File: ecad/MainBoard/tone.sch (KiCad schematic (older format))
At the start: 5 parts, among them IC1 RC4558

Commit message: Update BOM and SPIRCE SIM
Add netlist to calculate power dissipation through each resistor
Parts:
- C9: MPN (none) -> 12065C204KAT4A
- IC1: Digi-Key_PN (none) -> 296-9650-5-ND; MPN (none) -> RC4558D
- R11: Digi-Key_PN (none) -> PT220XTR-ND; MPN (none) -> ERJ-1TYJ221U
- R17: Digi-Key_PN (none) -> A130048TR-ND; MPN (none) -> CRGCQ0402J1K0
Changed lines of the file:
@@
 F 1 "220n" V 1000 1600 50  0000 C CNN
 F 2 "Capacitor_SMD:C_0805_2012Metric_Pad1.18x1.45mm_HandSolder" H 1188 1450 50  0001 C CNN
-F 3 "~" H 1150 1600 50  0001 C CNN
+F 3 "https://datasheets.avx.com/X7RDielectric.pdf" H 1150 1600 50  0001 C CNN
+F 4 "12065C204KAT4A" H 1150 1600 50  0001 C CNN "MPN"
 	1    1150 1600
 	0    -1   -1   0
@@
 F 2 "Resistor_SMD:R_0805_2012Metric_Pad1.20x1.40mm_HandSolder" V 1430 1600 50  0001 C CNN
 F 3 "~" H 1500 1600 50  0001 C CNN
+F 4 "PT220XTR-ND" H 1500 1600 50  0001 C CNN "Digi-Key_PN"
+F 5 "ERJ-1TYJ221U" H 1500 1600 50  0001 C CNN "MPN"
 	1    1500 1600
 	0    -1   -1   0
@@
 F 2 "Resistor_SMD:R_0805_2012Metric_Pad1.20x1.40mm_HandSolder" V 1530 1200 50  0001 C CNN
 F 3 "~" H 1600 1200 50  0001 C CNN
+F 4 "A130048TR-ND" H 1600 1200 50  0001 C CNN "Digi-Key_PN"
+F 5 "CRGCQ0402J1K0" H 1600 1200 50  0001 C CNN "MPN"
 	1    1600 1200
 	0    1    1    0
@@
 F 6 "Y" H 1550 850 50  0001 C CNN "Spice_Netlist_Enabled"
 F 7 "../lib/spice_models/RC4558.301.lib" H 1550 850 50  0001 C CNN "Spice_Lib_File"
+F 8 "296-9650-5-ND" H 1550 850 50  0001 C CNN "Digi-Key_PN"
+F 9 "RC4558D" H 1550 850 50  0001 C CNN "MPN"
 	2    1550 850
 	1    0    0    -1

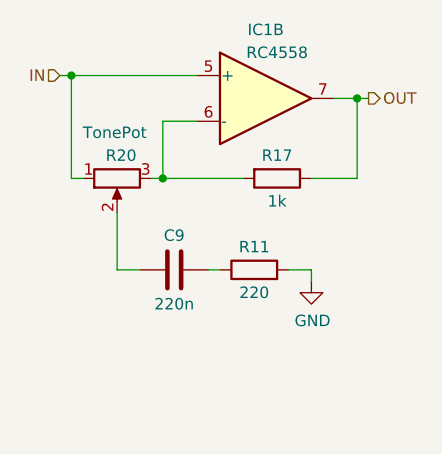
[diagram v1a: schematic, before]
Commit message: Clean up ecad
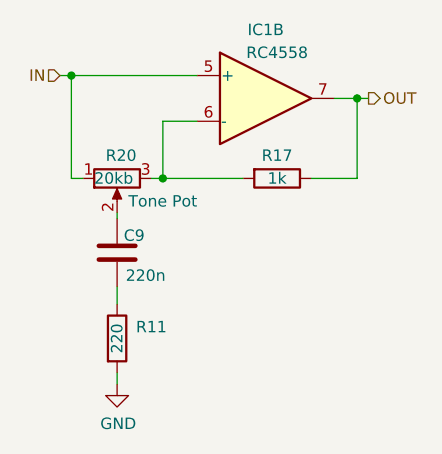
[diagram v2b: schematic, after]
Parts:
- C9: footprint Capacitor_SMD:C_0805_2012Metric_Pad1.18x1.45mm_HandSolder -> Capacitor_SMD:C_1206_3216Metric_Pad1.33x1.80mm_HandSolder; Digi-Key_PN (none) -> 478-12065C204KAT4ADKR-ND
- IC1: footprint Package_SO:Texas_R-PDSO-G8_EP2.95x4.9mm_Mask2.4x3.1mm -> DigiKey:SOIC-8_W3.9mm
- R11: footprint Resistor_SMD:R_0805_2012Metric_Pad1.20x1.40mm_HandSolder -> Resistor_SMD:R_2512_6332Metric_Pad1.40x3.35mm_HandSolder
- R17: footprint Resistor_SMD:R_0805_2012Metric_Pad1.20x1.40mm_HandSolder -> Resistor_SMD:R_0402_1005Metric_Pad0.72x0.64mm_HandSolder
- R20: value TonePot -> 20kb; Category (none) -> Tone Pot; Digi-Key_PN (none) -> 75160-195-08LF; Spice_Lib_File ../lib/spice_models/pot.lib -> ../lib/spice_models/pots.lib
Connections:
- net at R20.2: now also C9.2; no longer C9.1
- net at R11.1: now also C9.1; no longer C9.2
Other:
- moved on the sheet: C9, R11
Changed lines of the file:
@@
 encoding utf-8
 Sheet 3 5
-Title "Effects Board"
-Date "2021-01-17"
-Rev "1.0"
-Comp "Panda Pals"
-Comment1 "John McAvoy"
+Title "Screaming Panda Guitar Pedal"
+Date "2021-08-08"
+Rev "1v0"
+Comp "John McAvoy"
+Comment1 ""
 Comment2 ""
 Comment3 ""
@@
 L Device:C C?
 U 1 1 6027E33E
-P 1150 1600
+P 900 1525
 AR Path="/6027E33E" Ref="C?"  Part="1"
 AR Path="/60307048/6027E33E" Ref="C9"  Part="1"
-F 0 "C9" V 1300 1600 50  0000 C CNN
-F 1 "220n" V 1000 1600 50  0000 C CNN
-F 2 "Capacitor_SMD:C_0805_2012Metric_Pad1.18x1.45mm_HandSolder" H 1188 1450 50  0001 C CNN
-F 3 "https://datasheets.avx.com/X7RDielectric.pdf" H 1150 1600 50  0001 C CNN
-F 4 "12065C204KAT4A" H 1150 1600 50  0001 C CNN "MPN"
-	1    1150 1600
-	0    -1   -1   0
+F 0 "C9" H 825 1450 50  0000 C CNN
+F 1 "220n" H 775 1625 50  0000 C CNN
+F 2 "Capacitor_SMD:C_1206_3216Metric_Pad1.33x1.80mm_HandSolder" H 938 1375 50  0001 C CNN
+F 3 "https://datasheets.avx.com/X7RDielectric.pdf" H 900 1525 50  0001 C CNN
+F 4 "12065C204KAT4A" H 900 1525 50  0001 C CNN "MPN"
+F 5 "478-12065C204KAT4ADKR-ND" H 900 1525 50  0001 C CNN "Digi-Key_PN"
+	1    900  1525
+	-1   0    0    1
 $EndComp
 $Comp
 L Device:R R?
 U 1 1 6027E344
-P 1500 1600
+P 900 1900
 AR Path="/6027E344" Ref="R?"  Part="1"
 AR Path="/60307048/6027E344" Ref="R11"  Part="1"
-F 0 "R11" V 1600 1600 50  0000 C CNN
-F 1 "220" V 1400 1600 50  0000 C CNN
-F 2 "Resistor_SMD:R_0805_2012Metric_Pad1.20x1.40mm_HandSolder" V 1430 1600 50  0001 C CNN
-F 3 "~" H 1500 1600 50  0001 C CNN
-F 4 "PT220XTR-ND" H 1500 1600 50  0001 C CNN "Digi-Key_PN"
-F 5 "ERJ-1TYJ221U" H 1500 1600 50  0001 C CNN "MPN"
-	1    1500 1600
-	0    -1   -1   0
+F 0 "R11" H 1050 1950 50  0000 C CNN
+F 1 "220" V 900 1900 50  0000 C CNN
+F 2 "Resistor_SMD:R_2512_6332Metric_Pad1.40x3.35mm_HandSolder" V 830 1900 50  0001 C CNN
+F 3 "https://b2b-api.panasonic.eu/file_stream/pids/fileversion/1242" H 900 1900 50  0001 C CNN
+F 4 "PT220XTR-ND" H 900 1900 50  0001 C CNN "Digi-Key_PN"
+F 5 "ERJ-1TYJ221U" H 900 1900 50  0001 C CNN "MPN"
+	1    900  1900
+	1    0    0    -1
 $EndComp
-Wire Wire Line
-	1300 1600 1350 1600
 Text HLabel 2000 850  2    50   Output ~ 0
 OUT
@@
 AR Path="/60307048/6027E362" Ref="R17"  Part="1"
 F 0 "R17" V 1500 1200 50  0000 C CNN
-F 1 "1k" V 1700 1200 50  0000 C CNN
-F 2 "Resistor_SMD:R_0805_2012Metric_Pad1.20x1.40mm_HandSolder" V 1530 1200 50  0001 C CNN
-F 3 "~" H 1600 1200 50  0001 C CNN
+F 1 "1k" V 1600 1200 50  0000 C CNN
+F 2 "Resistor_SMD:R_0402_1005Metric_Pad0.72x0.64mm_HandSolder" V 1530 1200 50  0001 C CNN
+F 3 "https://www.te.com/commerce/DocumentDelivery/DDEController?Action=srchrtrv&DocNm=1773204-3&DocType=DS&DocLang=English" H 1600 1200 50  0001 C CNN
 F 4 "A130048TR-ND" H 1600 1200 50  0001 C CNN "Digi-Key_PN"
 F 5 "CRGCQ0402J1K0" H 1600 1200 50  0001 C CNN "MPN"
@@
 F 0 "IC1" H 1550 1150 50  0000 C CNN
 F 1 "RC4558" H 1600 1050 50  0000 C CNN
-F 2 "Package_SO:Texas_R-PDSO-G8_EP2.95x4.9mm_Mask2.4x3.1mm" H 1550 850 50  0001 C CNN
+F 2 "DigiKey:SOIC-8_W3.9mm" H 1550 850 50  0001 C CNN
 F 3 "http://www.ti.com/lit/ds/symlink/rc4558.pdf" H 1550 850 50  0001 C CNN
 F 4 "X" H 1550 850 50  0001 C CNN "Spice_Primitive"
@@
 P 900 1200
 F 0 "R20" V 800 1250 50  0000 R CNN
-F 1 "TonePot" V 700 1350 50  0000 R CNN
+F 1 "20kb" V 900 1300 50  0000 R CNN
 F 2 "Connector_PinHeader_2.54mm:PinHeader_1x03_P2.54mm_Vertical" H 900 1200 50  0001 C CNN
-F 3 "~" H 900 1200 50  0001 C CNN
+F 3 "https://www.bourns.com/docs/Product-Datasheets/PTV09.pdf" H 900 1200 50  0001 C CNN
 F 4 "X" H 900 1200 50  0001 C CNN "Spice_Primitive"
 F 5 "POTTone" H 900 1200 50  0001 C CNN "Spice_Model"
 F 6 "Y" H 900 1200 50  0001 C CNN "Spice_Netlist_Enabled"
-F 7 "../lib/spice_models/pot.lib" H 900 1200 50  0001 C CNN "Spice_Lib_File"
+F 7 "../lib/spice_models/pots.lib" H 900 1200 50  0001 C CNN "Spice_Lib_File"
+F 8 "Tone Pot" V 1000 1000 50  0000 C CNN "Category"
+F 9 "75160-195-08LF" H 900 1200 50  0001 C CNN "Digi-Key_PN"
+F 10 "" H 900 1200 50  0001 C CNN "MPN"
 	1    900  1200
 	0    -1   1    0
@@
 L power:GND #PWR?
 U 1 1 6027E34B
-P 1750 1650
+P 900 2100
 AR Path="/6027E34B" Ref="#PWR?"  Part="1"
 AR Path="/60307048/6027E34B" Ref="#PWR017"  Part="1"
-F 0 "#PWR017" H 1750 1400 50  0001 C CNN
-F 1 "GND" H 1755 1477 50  0000 C CNN
-F 2 "" H 1750 1650 50  0001 C CNN
-F 3 "" H 1750 1650 50  0001 C CNN
-	1    1750 1650
+F 0 "#PWR017" H 900 1850 50  0001 C CNN
+F 1 "GND" H 905 1927 50  0000 C CNN
+F 2 "" H 900 2100 50  0001 C CNN
+F 3 "" H 900 2100 50  0001 C CNN
+	1    900  2100
 	1    0    0    -1
 $EndComp
 Wire Wire Line
-	1750 1650 1750 1600
-Wire Wire Line
-	1650 1600 1750 1600
-Wire Wire Line
-	900  1350 900  1600
-Wire Wire Line
-	900  1600 1000 1600
+	900  1350 900  1375
 Wire Wire Line
 	1050 1200 1100 1200
@@
 Wire Wire Line
 	700  750  1250 750
+Wire Wire Line
+	900  2100 900  2050
+Wire Wire Line
+	900  1750 900  1675
 $EndSCHEMATC

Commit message: Update ecad BOM
Change transistor to 2N4424
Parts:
- C9: footprint Capacitor_SMD:C_1206_3216Metric_Pad1.33x1.80mm_HandSolder -> Capacitor_SMD:C_0805_2012Metric_Pad1.18x1.45mm_HandSolder; MPN 12065C204KAT4A -> C0805C224K5RACTU
- R11: footprint Resistor_SMD:R_2512_6332Metric_Pad1.40x3.35mm_HandSolder -> Resistor_SMD:R_0805_2012Metric_Pad1.20x1.40mm_HandSolder; MPN ERJ-1TYJ221U -> ERJ-6GEYJ221V
- R17: footprint Resistor_SMD:R_0402_1005Metric_Pad0.72x0.64mm_HandSolder -> Resistor_SMD:R_0805_2012Metric_Pad1.20x1.40mm_HandSolder; MPN CRGCQ0402J1K0 -> ERA6AEB102V
- R20: footprint Connector_PinHeader_2.54mm:PinHeader_1x03_P2.54mm_Vertical -> DigiKey:PinHeader_1x3_P2.54_Drill1.1mm; MPN (none) -> 0901200160
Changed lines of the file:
@@
 F 0 "C9" H 825 1450 50  0000 C CNN
 F 1 "220n" H 775 1625 50  0000 C CNN
-F 2 "Capacitor_SMD:C_1206_3216Metric_Pad1.33x1.80mm_HandSolder" H 938 1375 50  0001 C CNN
-F 3 "https://datasheets.avx.com/X7RDielectric.pdf" H 900 1525 50  0001 C CNN
-F 4 "12065C204KAT4A" H 900 1525 50  0001 C CNN "MPN"
+F 2 "Capacitor_SMD:C_0805_2012Metric_Pad1.18x1.45mm_HandSolder" H 938 1375 50  0001 C CNN
+F 3 "https://datasheet.octopart.com/C0805C224K5RACTU-Kemet-datasheet-5313890.pdf" H 900 1525 50  0001 C CNN
+F 4 "C0805C224K5RACTU" H 900 1525 50  0001 C CNN "MPN"
 F 5 "478-12065C204KAT4ADKR-ND" H 900 1525 50  0001 C CNN "Digi-Key_PN"
 	1    900  1525
@@
 F 0 "R11" H 1050 1950 50  0000 C CNN
 F 1 "220" V 900 1900 50  0000 C CNN
-F 2 "Resistor_SMD:R_2512_6332Metric_Pad1.40x3.35mm_HandSolder" V 830 1900 50  0001 C CNN
-F 3 "https://b2b-api.panasonic.eu/file_stream/pids/fileversion/1242" H 900 1900 50  0001 C CNN
+F 2 "Resistor_SMD:R_0805_2012Metric_Pad1.20x1.40mm_HandSolder" V 830 1900 50  0001 C CNN
+F 3 "https://datasheet.octopart.com/ERJ-6GEYJ221V-Panasonic-datasheet-13266872.pdf" H 900 1900 50  0001 C CNN
 F 4 "PT220XTR-ND" H 900 1900 50  0001 C CNN "Digi-Key_PN"
-F 5 "ERJ-1TYJ221U" H 900 1900 50  0001 C CNN "MPN"
+F 5 "ERJ-6GEYJ221V" H 900 1900 50  0001 C CNN "MPN"
 	1    900  1900
 	1    0    0    -1
@@
 F 0 "R17" V 1500 1200 50  0000 C CNN
 F 1 "1k" V 1600 1200 50  0000 C CNN
-F 2 "Resistor_SMD:R_0402_1005Metric_Pad0.72x0.64mm_HandSolder" V 1530 1200 50  0001 C CNN
-F 3 "https://www.te.com/commerce/DocumentDelivery/DDEController?Action=srchrtrv&DocNm=1773204-3&DocType=DS&DocLang=English" H 1600 1200 50  0001 C CNN
+F 2 "Resistor_SMD:R_0805_2012Metric_Pad1.20x1.40mm_HandSolder" V 1530 1200 50  0001 C CNN
+F 3 "https://datasheet.octopart.com/ERA6AEB102V-Panasonic-datasheet-62287448.pdf" H 1600 1200 50  0001 C CNN
 F 4 "A130048TR-ND" H 1600 1200 50  0001 C CNN "Digi-Key_PN"
-F 5 "CRGCQ0402J1K0" H 1600 1200 50  0001 C CNN "MPN"
+F 5 "ERA6AEB102V" H 1600 1200 50  0001 C CNN "MPN"
 	1    1600 1200
 	0    1    1    0
@@
 F 0 "R20" V 800 1250 50  0000 R CNN
 F 1 "20kb" V 900 1300 50  0000 R CNN
-F 2 "Connector_PinHeader_2.54mm:PinHeader_1x03_P2.54mm_Vertical" H 900 1200 50  0001 C CNN
-F 3 "https://www.bourns.com/docs/Product-Datasheets/PTV09.pdf" H 900 1200 50  0001 C CNN
+F 2 "DigiKey:PinHeader_1x3_P2.54_Drill1.1mm" H 900 1200 50  0001 C CNN
+F 3 "https://www.molex.com/pdm_docs/sd/901200160_sd.pdf" H 900 1200 50  0001 C CNN
 F 4 "X" H 900 1200 50  0001 C CNN "Spice_Primitive"
 F 5 "POTTone" H 900 1200 50  0001 C CNN "Spice_Model"
@@
 F 8 "Tone Pot" V 1000 1000 50  0000 C CNN "Category"
 F 9 "75160-195-08LF" H 900 1200 50  0001 C CNN "Digi-Key_PN"
-F 10 "" H 900 1200 50  0001 C CNN "MPN"
+F 10 "0901200160" H 900 1200 50  0001 C CNN "MPN"
 	1    900  1200
 	0    -1   1    0

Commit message: Library recovery
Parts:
- IC1: footprint DigiKey:SOIC-8_W3.9mm -> digikey-footprints:SOIC-8_W5.6mm
- R20: footprint DigiKey:PinHeader_1x3_P2.54_Drill1.1mm -> screaming-panda:75160-195-03LF
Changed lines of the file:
@@
 F 0 "IC1" H 1550 1150 50  0000 C CNN
 F 1 "RC4558" H 1600 1050 50  0000 C CNN
-F 2 "DigiKey:SOIC-8_W3.9mm" H 1550 850 50  0001 C CNN
+F 2 "digikey-footprints:SOIC-8_W5.6mm" H 1550 850 50  0001 C CNN
 F 3 "http://www.ti.com/lit/ds/symlink/rc4558.pdf" H 1550 850 50  0001 C CNN
 F 4 "X" H 1550 850 50  0001 C CNN "Spice_Primitive"
@@
 F 0 "R20" V 800 1250 50  0000 R CNN
 F 1 "20kb" V 900 1300 50  0000 R CNN
-F 2 "DigiKey:PinHeader_1x3_P2.54_Drill1.1mm" H 900 1200 50  0001 C CNN
+F 2 "screaming-panda:75160-195-03LF" H 900 1200 50  0001 C CNN
 F 3 "https://www.molex.com/pdm_docs/sd/901200160_sd.pdf" H 900 1200 50  0001 C CNN
 F 4 "X" H 900 1200 50  0001 C CNN "Spice_Primitive"

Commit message: Change to using kicad-library submodule
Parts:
- IC1: Spice_Lib_File ../lib/spice_models/RC4558.301.lib -> ../lib/kicad-library/spice_models/RC4558.301.lib
- R20: Spice_Lib_File ../lib/spice_models/pots.lib -> ../lib/kicad-library/spice_models/pots.lib
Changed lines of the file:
@@
 F 5 "RC4558" H 1550 850 50  0001 C CNN "Spice_Model"
 F 6 "Y" H 1550 850 50  0001 C CNN "Spice_Netlist_Enabled"
-F 7 "../lib/spice_models/RC4558.301.lib" H 1550 850 50  0001 C CNN "Spice_Lib_File"
+F 7 "../lib/kicad-library/spice_models/RC4558.301.lib" H 1550 850 50  0001 C CNN "Spice_Lib_File"
 F 8 "296-9650-5-ND" H 1550 850 50  0001 C CNN "Digi-Key_PN"
 F 9 "RC4558D" H 1550 850 50  0001 C CNN "MPN"
@@
 F 5 "POTTone" H 900 1200 50  0001 C CNN "Spice_Model"
 F 6 "Y" H 900 1200 50  0001 C CNN "Spice_Netlist_Enabled"
-F 7 "../lib/spice_models/pots.lib" H 900 1200 50  0001 C CNN "Spice_Lib_File"
+F 7 "../lib/kicad-library/spice_models/pots.lib" H 900 1200 50  0001 C CNN "Spice_Lib_File"
 F 8 "Tone Pot" V 1000 1000 50  0000 C CNN "Category"
 F 9 "75160-195-08LF" H 900 1200 50  0001 C CNN "Digi-Key_PN"
